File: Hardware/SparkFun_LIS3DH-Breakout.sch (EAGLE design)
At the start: 15 parts, among them U2 LIS3DH

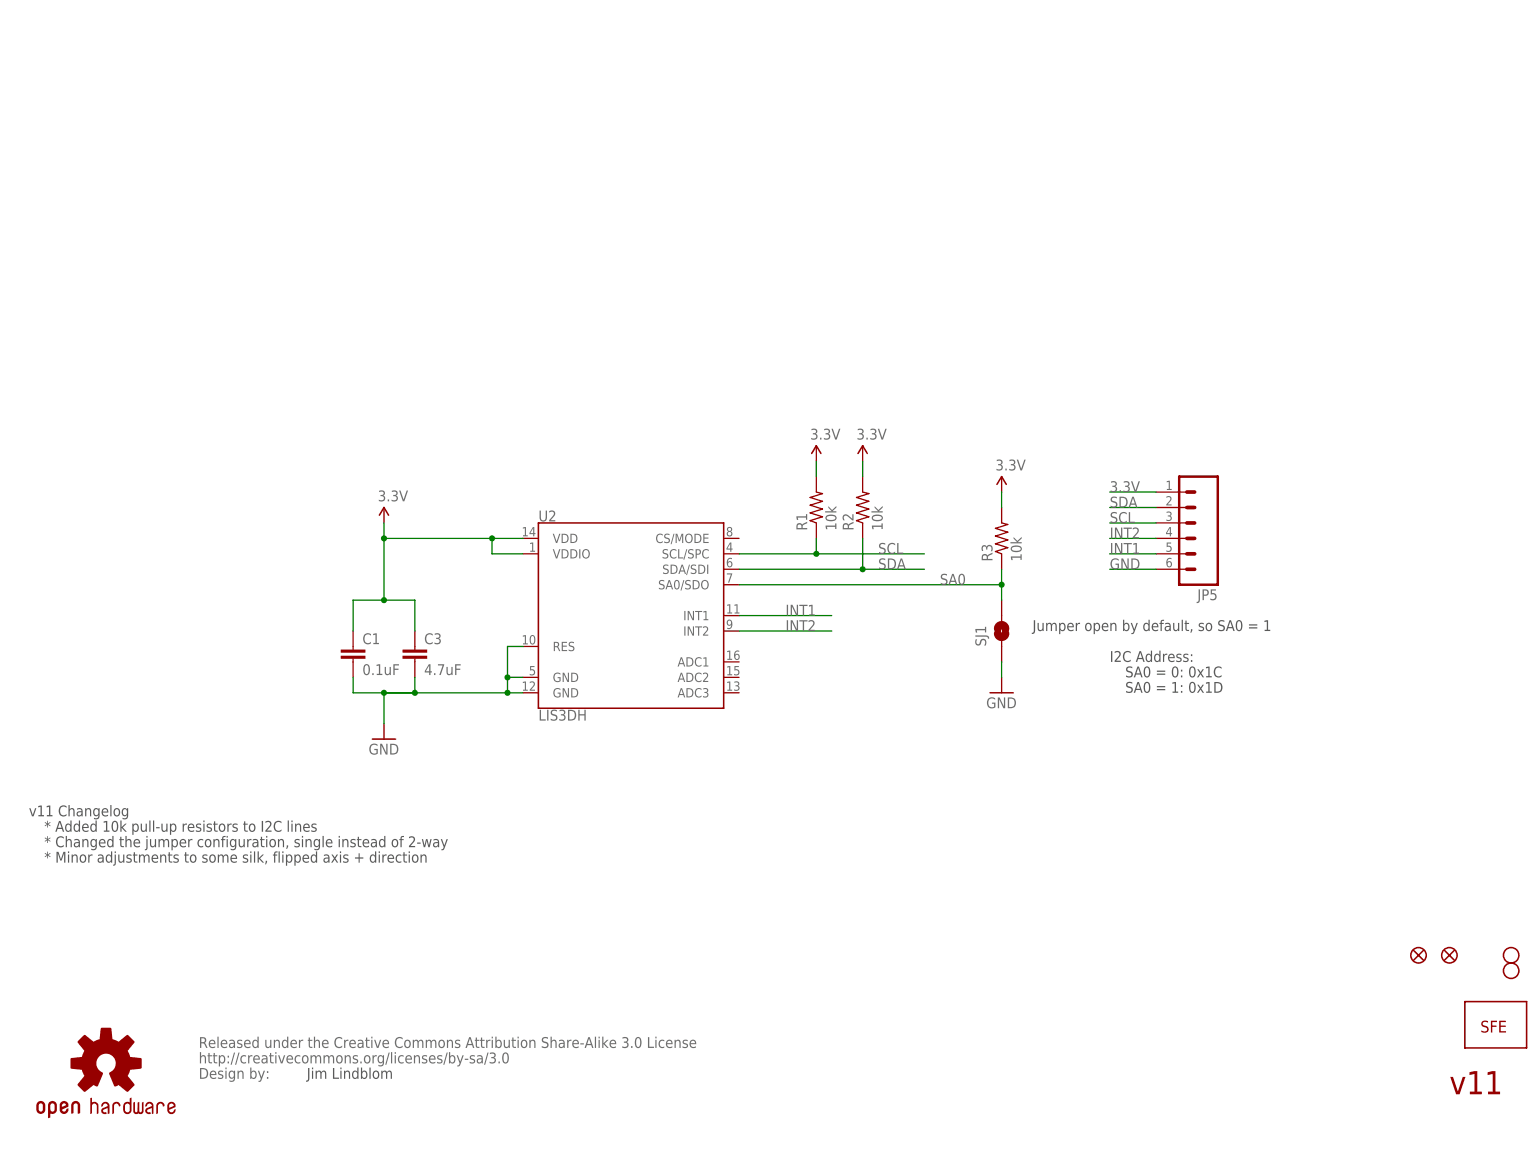
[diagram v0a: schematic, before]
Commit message: Finished design for proto 1
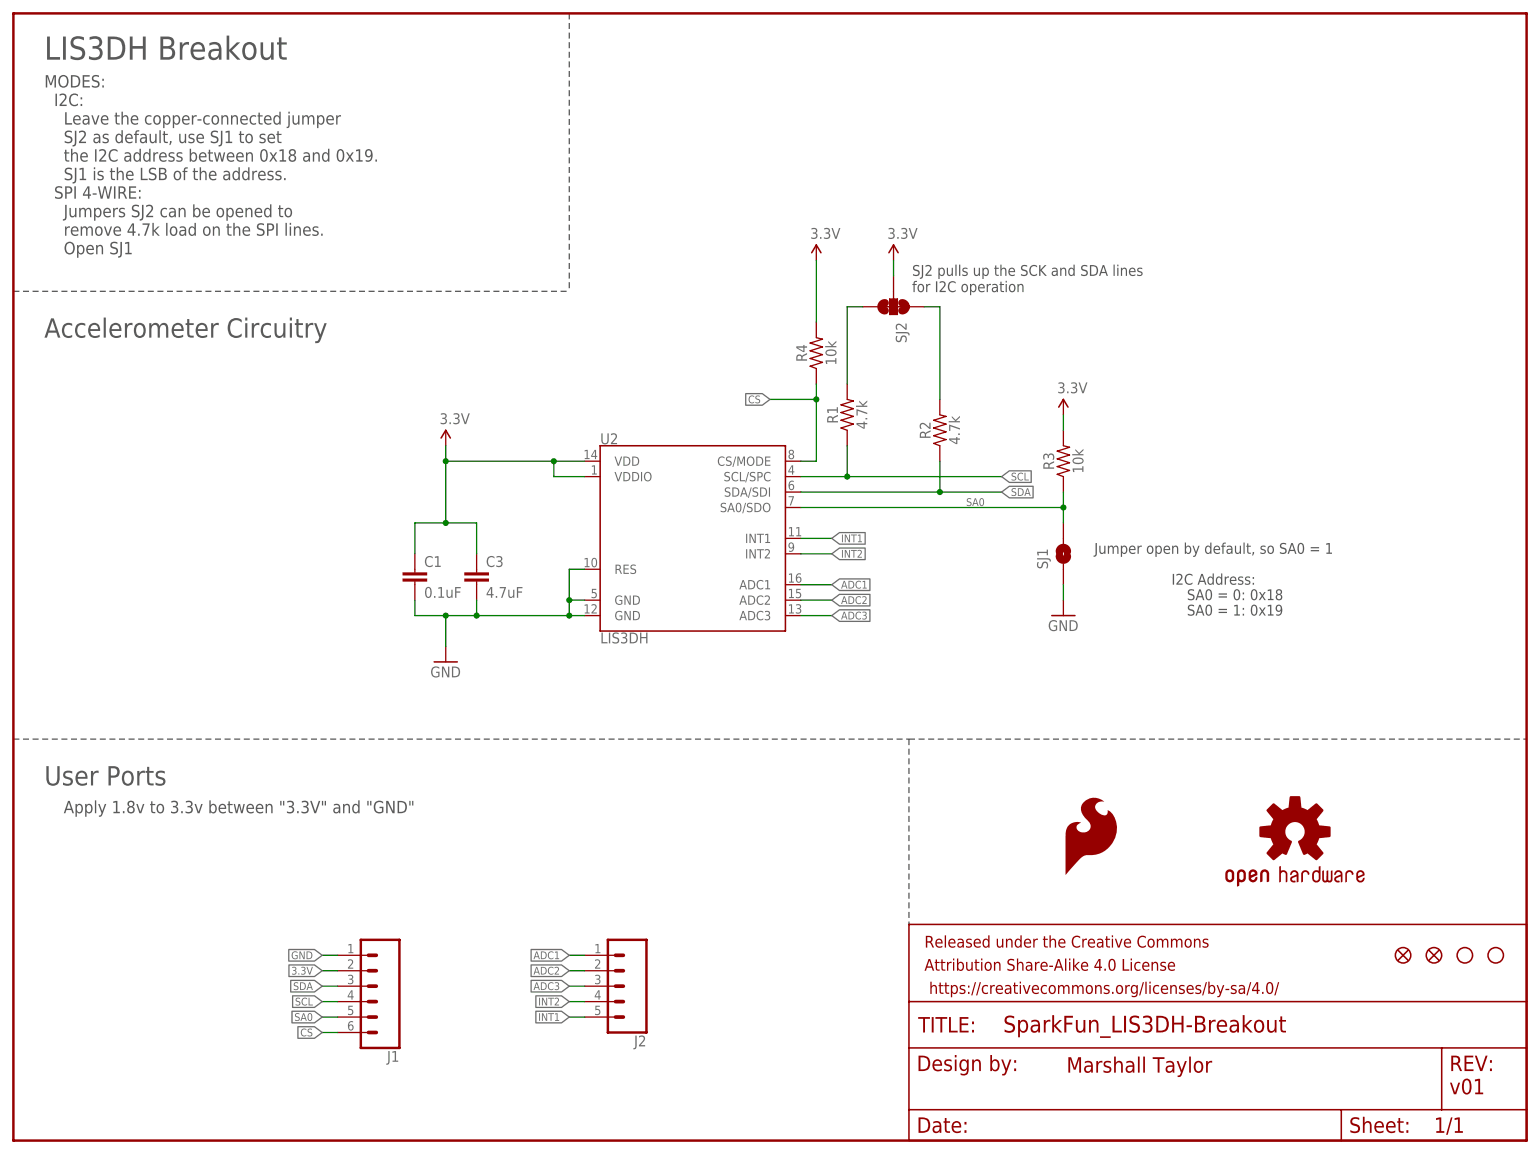
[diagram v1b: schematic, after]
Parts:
- removed JP1: LOGO-SFESK, SparkFun:LOGO-SFESK
- removed JP5: (no value), SparkFun:M06SIP
- removed U$2: CREATIVE_COMMONS, SparkFun:CREATIVE_COMMONS
- added FRAME2: FRAME-LETTER, SparkFun-Aesthetics:FRAME-LETTER
- added J1: (no value), SparkFun-Connectors:CONN_06SILK_FEMALE_PTH
- added J2: (no value), SparkFun-Connectors:CONN_05PTH
- added LOGO1: SFE_LOGO_FLAME.1_INCH, SparkFun-Aesthetics:SFE_LOGO_FLAME.1_INCH
- added R4: 10k, SparkFun-Resistors:10KOHM-0603-1/10W-1%
- added SJ2: (no value), TestAperatures:JUMPER-PAD-3-NC_BY_TRACE
- R1, R2: value 10k -> 4.7k; device SparkFun:RESISTOR0402-RES -> SparkFun-Resistors:4.7KOHM-0603-1/10W-1%
- R3: device SparkFun:RESISTOR0402-RES -> SparkFun-Resistors:10KOHM-0603-1/10W-1%
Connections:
- new net ADC1: J2.1, U2.ADC1
- new net ADC2: J2.2, U2.ADC2
- new net ADC3: J2.3, U2.ADC3
- new net CS: J1.6, R4.1, U2.CS/MODE
- new net N$1: R2.2, SJ2.1
- new net N$2: R1.2, SJ2.3
- net 3.3V: now also J1.2, R4.2, SJ2.2; no longer JP5.1, R1.2, R2.2
- net GND: now also J1.1; no longer JP5.6
- net INT1: now also J2.5; no longer JP5.5
- net INT2: now also J2.4; no longer JP5.4
- net SA0: now also J1.5
- net SCL: now also J1.4; no longer JP5.3
- net SDA: now also J1.3; no longer JP5.2
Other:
- note added: "Accelerometer Circuitry"
- note added: "Apply 1.8v to 3.3v between "3.3V" and "GND""
- note added: "LIS3DH Breakout"
- note added: "MODES: I2C: Leave the copper-connected jumper SJ2 as default, use SJ1 to set the I2C address between 0x18 and 0x19. SJ1 is the LSB of the address. SPI 4-WIRE: Jumpers SJ2 can be opened to remove 4.7k load on the SPI lines. Open SJ1"
- note added: "Marshall Taylor"
- note added: "SA0 = 0: 0x18"
- note added: "SA0 = 1: 0x19"
- note added: "SJ2 pulls up the SCK and SDA lines for I2C operation"
- note added: "User Ports"
- note added: "v01"
- note removed: "* Added 10k pull-up resistors to I2C lines"
- note removed: "* Changed the jumper configuration, single instead of 2-way"
- note removed: "* Minor adjustments to some silk, flipped axis + direction"
- note removed: "Jim Lindblom"
- note removed: "SA0 = 0: 0x1C"
- note removed: "SA0 = 1: 0x1D"
- note removed: "v11"
- note removed: "v11 Changelog"
- moved on the sheet: C1, C3, R1, R2, R3, SJ1, U2
